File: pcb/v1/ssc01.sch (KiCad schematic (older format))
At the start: 21 parts, among them J1 UART, SW1 Reset, U1 74HCT04, U2 MC68B50, U3 74LS32, U4 Z80CPU, U5 SST39SF040, U6 62256, Y1 7.3728Hz

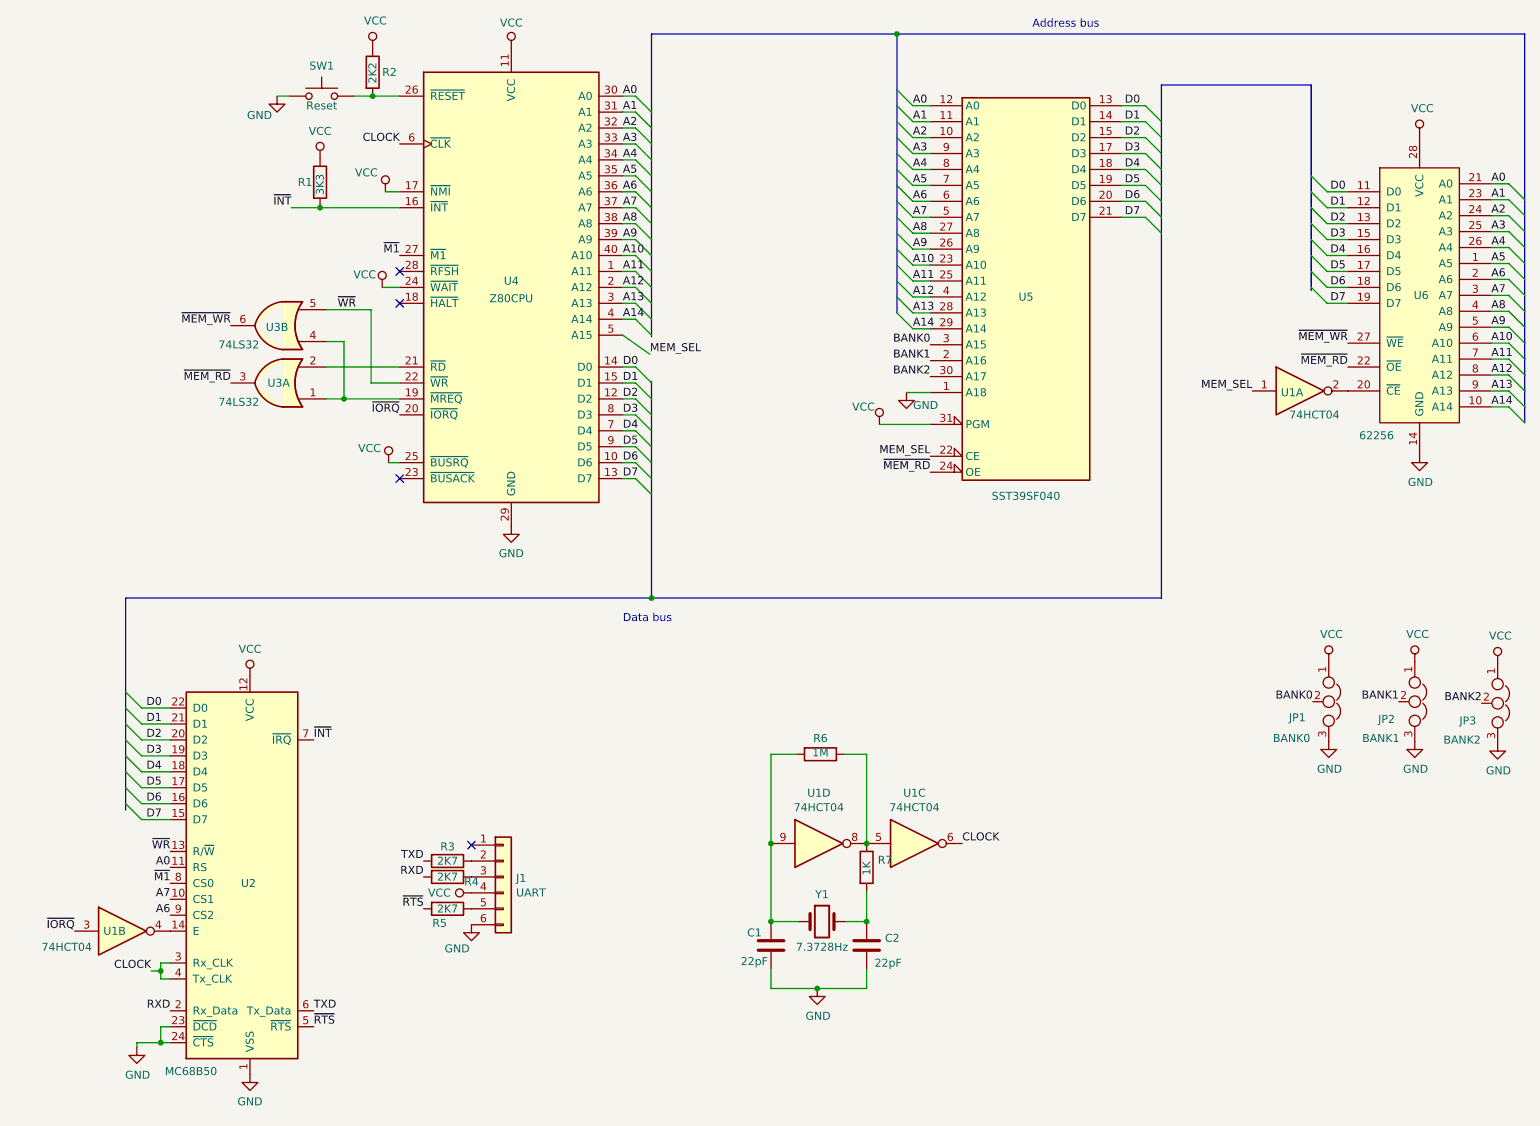
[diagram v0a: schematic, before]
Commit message: minor pcb changes
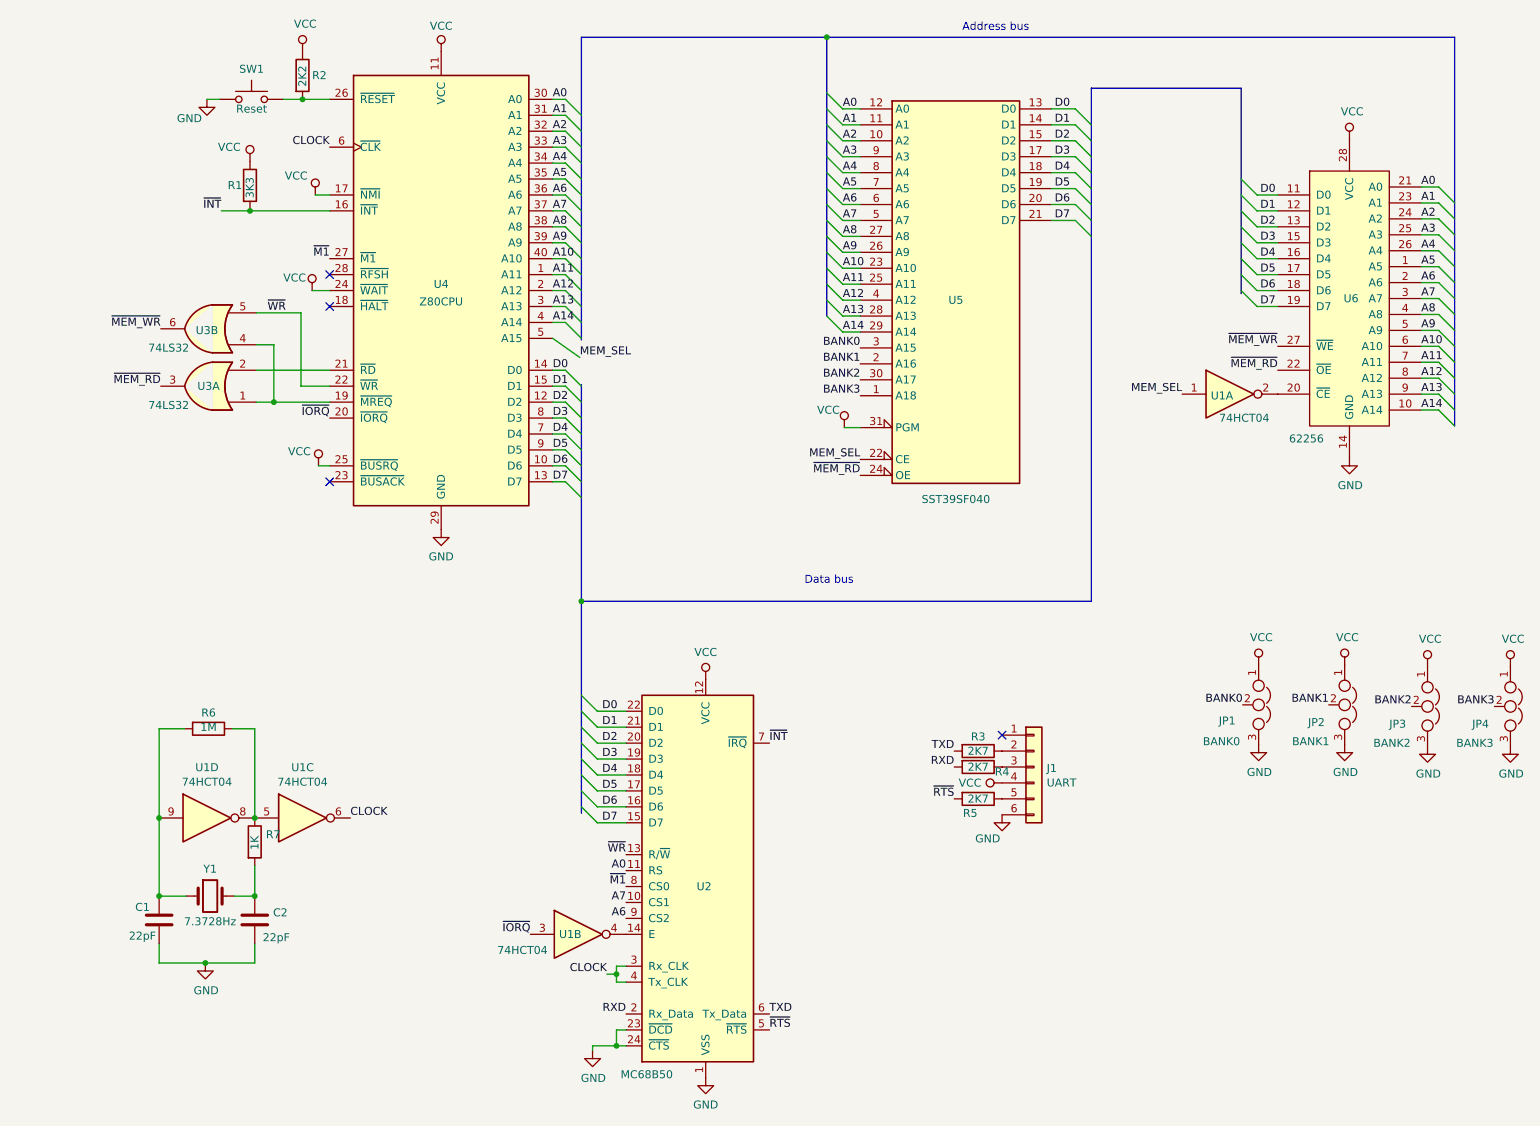
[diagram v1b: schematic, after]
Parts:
- added JP4: BANK3, symbol Device:Jumper_NC_Dual
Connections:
- net GND: now also JP4.3; no longer U5.1 (A18)
- net VCC: now also JP4.1
- new net BANK3: JP4.2, U5.1 (A18)
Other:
- moved on the sheet: C1, C2, J1, JP1, JP2, JP3, R1, R2, R3, R4, R5, R6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
